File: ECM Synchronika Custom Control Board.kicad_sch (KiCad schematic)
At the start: 0 parts

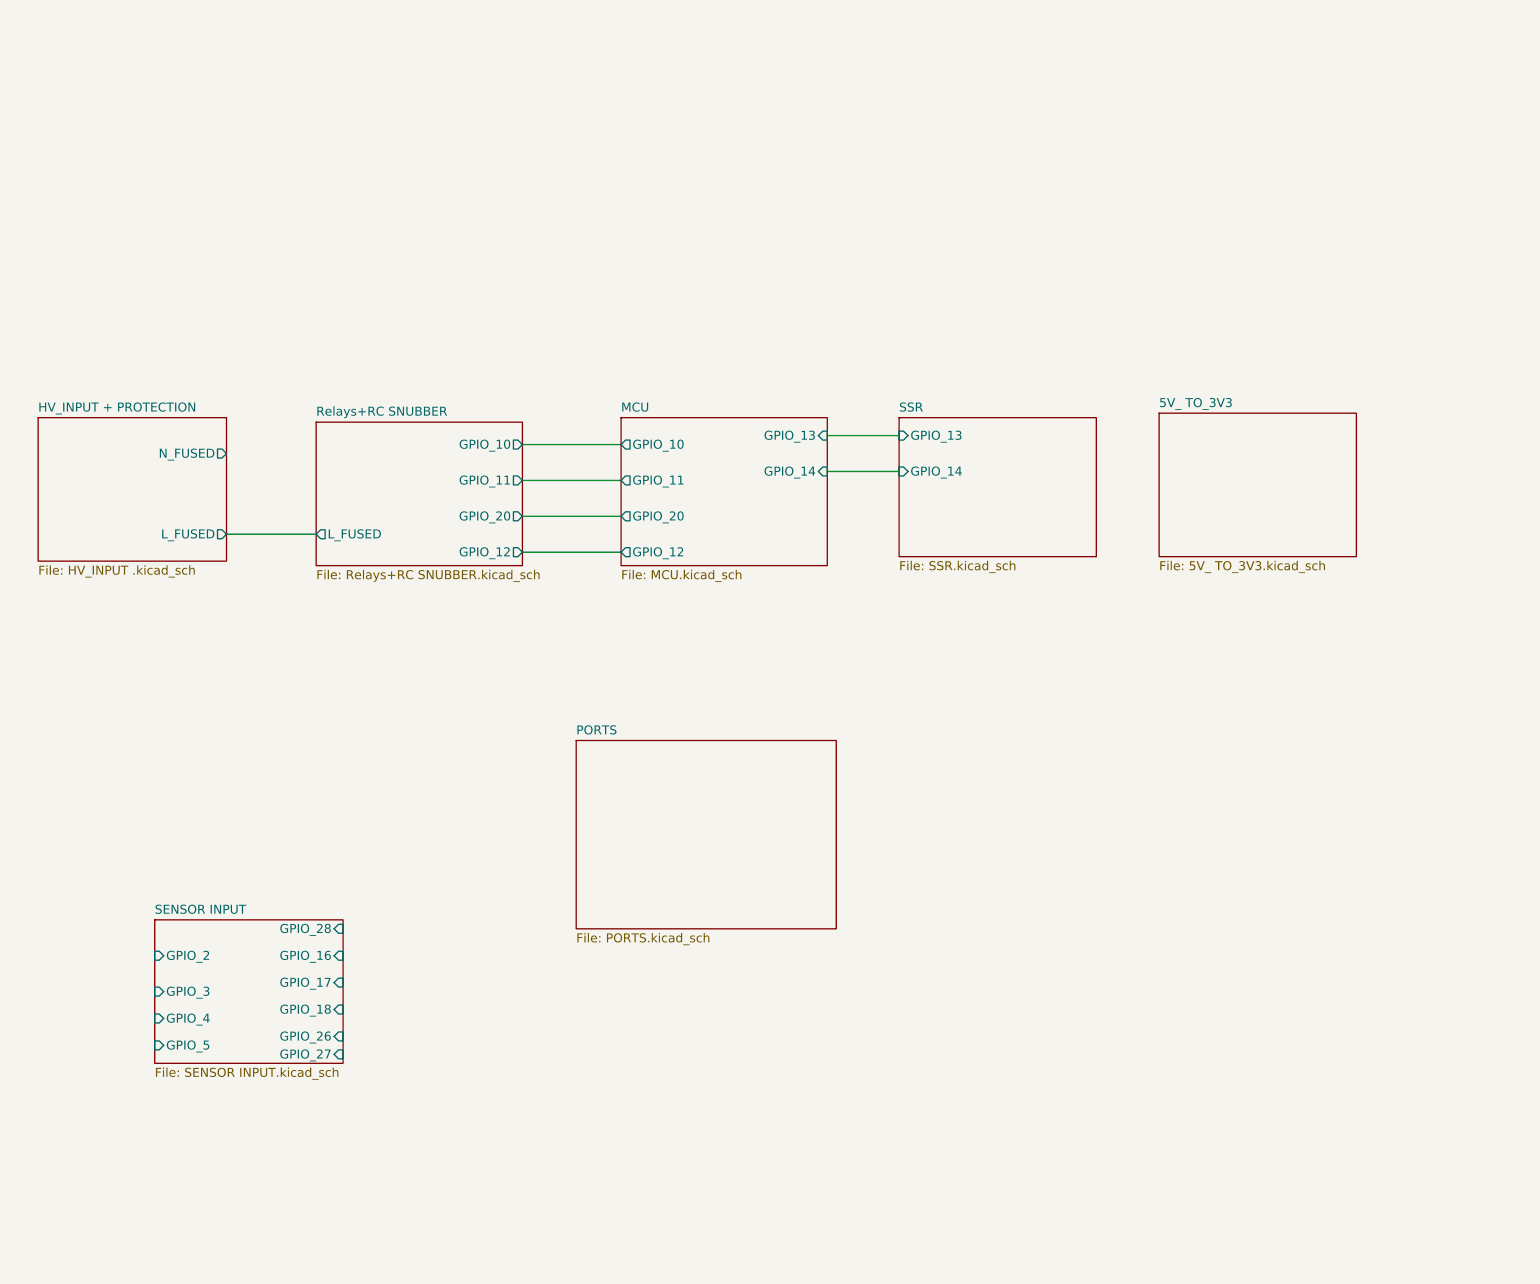
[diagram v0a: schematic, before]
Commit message: Update KiCad project files
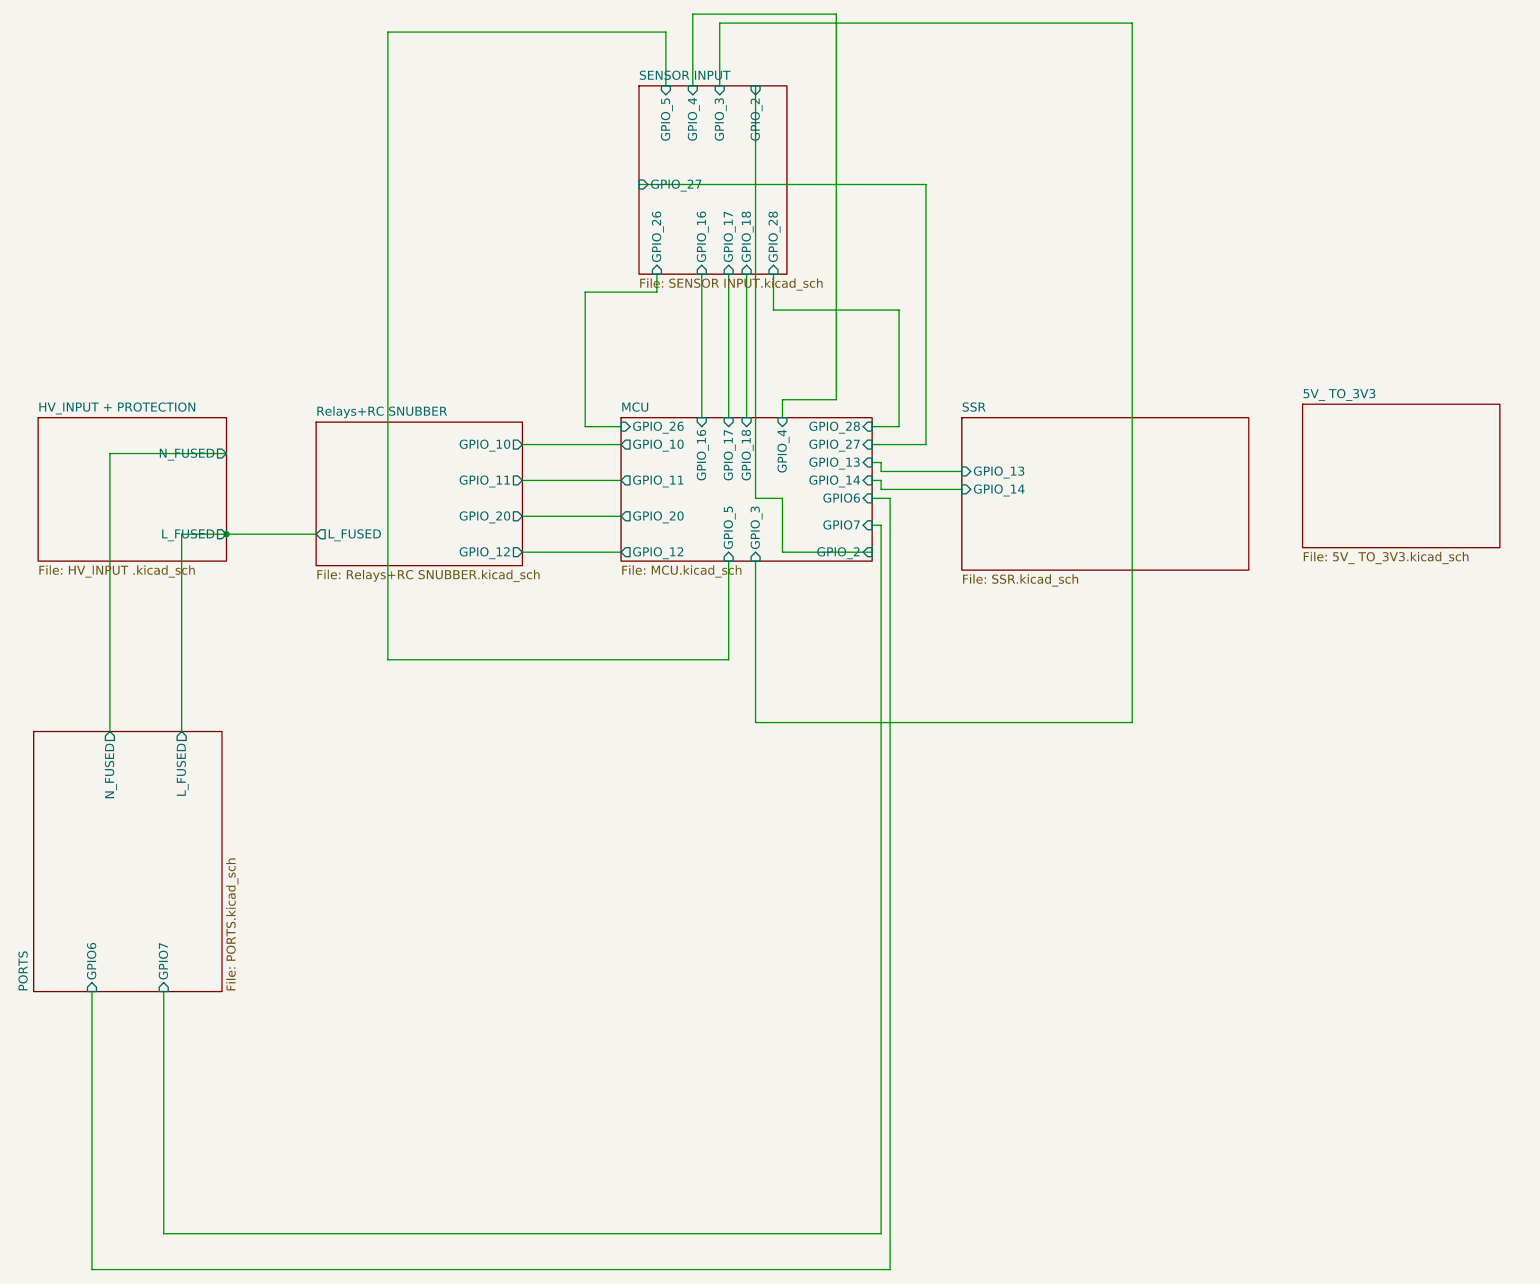
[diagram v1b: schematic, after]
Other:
- sheet MCU ports: added GPIO6, GPIO7, GPIO_16, GPIO_17, GPIO_18, GPIO_2, GPIO_26, GPIO_27, GPIO_28, GPIO_3, GPIO_4, GPIO_5; removed none
- sheet PORTS ports: added GPIO6, GPIO7, L_FUSED, N_FUSED; removed none
